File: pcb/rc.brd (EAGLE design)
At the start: 64.8 x 69.2 mm, 79 parts, among them IC2 TP4056

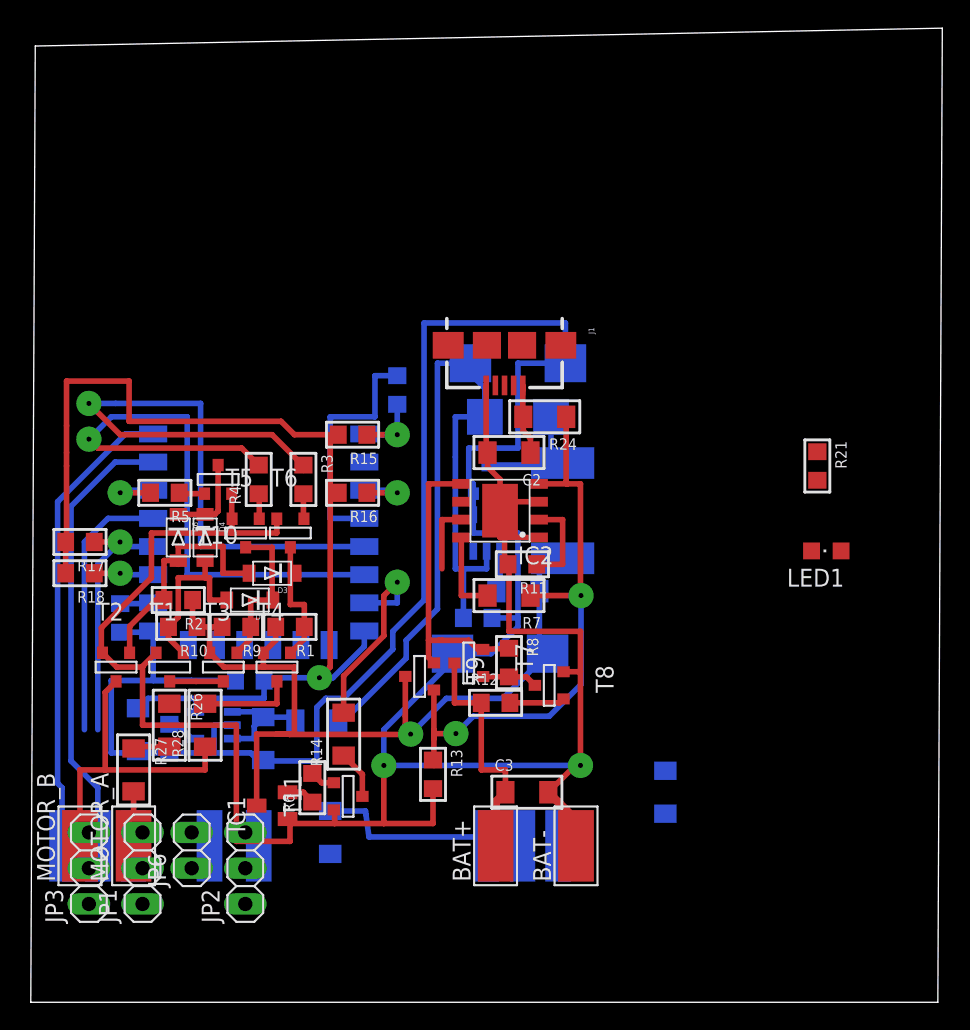
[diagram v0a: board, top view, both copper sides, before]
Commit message: pcb
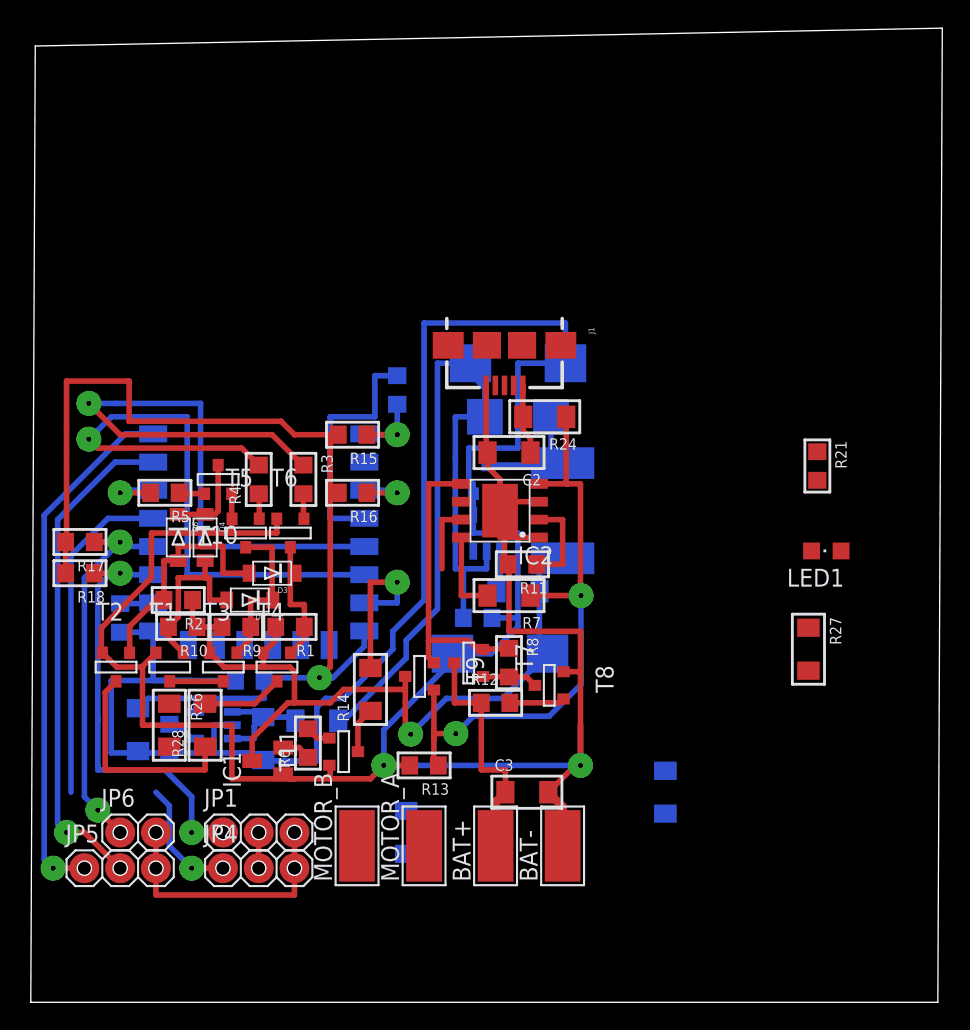
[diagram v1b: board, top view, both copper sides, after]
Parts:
- removed FLASH1, FLASH2, GND, RX, SERVO_CONTROL, SERVO_GND, SERVO_POWER, TX: WIREPADSMD5-1,8, wirepad:5-1,8
- removed JP2, JP3: (no value), pinhead:1X03
- added JP4, JP5: (no value), my:1X03
- JP1: device pinhead:1X03 -> my:1X03
- JP6: device pinhead:1X02 -> my:1X02
- moved R27 48.7 mm to (53.3, 19.7)
- moved MOTOR_A 20.6 mm to (26.0, 5.71)
- moved MOTOR_B 19.7 mm to (21.3, 5.71)
- moved JP1 8.64 mm to (14.3, 6.67), turned to 0 degrees
- moved R22 5.40 mm to (24.8, 6.67), turned to 90 degrees
- moved JP6 4.02 mm to (5.71, 6.67), turned to 0 degrees
- moved R14 3.70 mm to (22.2, 16.8)
- moved IC1 3.19 mm to (14.9, 11.7)
- moved R6 3.19 mm to (17.8, 13.0)
- moved T11 3.19 mm to (20.3, 12.4)
- moved BAT- 0.95 mm to (35.9, 5.71)
- moved R13 0.90 mm to (26.0, 11.4), turned to 180 degrees
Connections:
- net SERVO_CONTROL renamed SERVO#1_CTRL
- removed net N$29: R22.1, SERVO_CONTROL.1
- new net SERVO#2_CTRL: JP1.1, R18.1, U1.GPIO2
- net 5V: now also JP1.2
- net GND: now also JP1.3, JP4.3, JP5.3, JP6.2; no longer FLASH2.1, GND.1, SERVO_GND.1
- net N$21: now also JP6.1; no longer FLASH1.1
- net N$22: now also JP4.1, R22.1; no longer R18.1, U1.GPIO2
- net N$30: now also JP4.2; no longer SERVO_POWER.1
- net RX: now also JP5.2; no longer RX.1
- net TX: now also JP5.1; no longer TX.1
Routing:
- net SERVO#2_CTRL: track 0.00 -> 31.8 mm, vias 0 -> 2
- net N$29: track 13.4 -> 0.00 mm
- net N$21: track 19.3 -> 28.1 mm, vias 1 -> 2
- net N$4: track 23.4 -> 16.3 mm
- net BAT_PROT: track 62.3 -> 56.9 mm
- net SERVO#1_CTRL: track 18.9 -> 23.8 mm
- net N$22: track 4.29 -> 8.67 mm
- net TX: track 33.4 -> 37.7 mm, vias 0 -> 1
- net N$36: track 3.87 -> 0.00 mm
- net RX: track 32.1 -> 35.8 mm, vias 0 -> 1
- net BAT_CHECK: track 14.7 -> 11.8 mm
- net N$35: track 2.67 -> 0.13 mm
- net N$30: track 0.00 -> 2.54 mm
- net N$37: track 6.69 -> 5.76 mm
- net GND: track 277.1 -> 277.8 mm
